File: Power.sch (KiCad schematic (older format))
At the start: 13 parts, among them P1 24 Pin Mini-Fit Jr, SW1 Power Switch

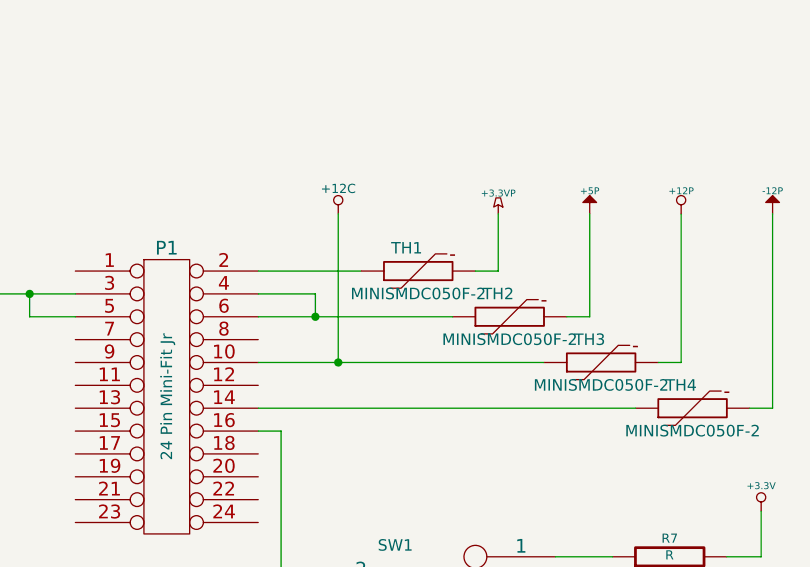
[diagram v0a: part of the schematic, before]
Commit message: Layout sessions 1-4.
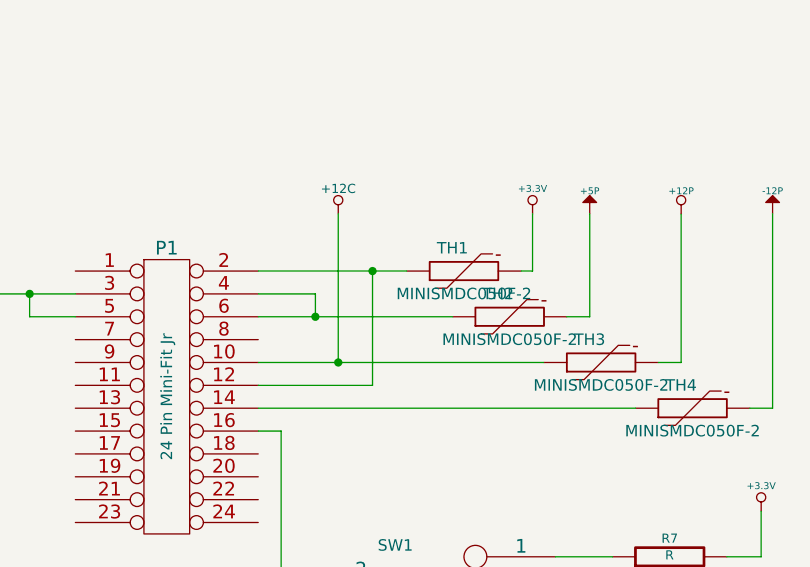
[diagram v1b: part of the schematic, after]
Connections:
- net +3.3VP is gone; now on net +3.3V: TH1.2
- net at P1.12 (P12): now also P1.2 (P2), TH1.1
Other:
- moved on the sheet: TH1
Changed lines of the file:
@@
 $EndComp
 Wire Wire Line
-	3250 2550 3700 2550
-Wire Wire Line
-	4200 2550 4300 2550
-Wire Wire Line
-	4300 2550 4300 2300
+	3250 2550 3900 2550
+Wire Wire Line
+	4400 2550 4450 2550
+Wire Wire Line
+	4450 2550 4450 2300
 Wire Wire Line
 	3250 2650 3500 2650
@@
 L THERMISTOR TH1
 U 1 1 52F96A4C
-P 3950 2550
-F 0 "TH1" V 4050 2600 50  0000 C CNN
-F 1 "MINISMDC050F-2" V 3850 2550 50  0000 C CNN
-F 2 "" H 3950 2550 60  0000 C CNN
-F 3 "" H 3950 2550 60  0000 C CNN
-F 4 "TE Connectivity" H 3950 2550 60  0001 C CNN "MFG name"
-F 5 "MINISMDC050F-2" H 3950 2550 60  0001 C CNN "MFG Part Number"
-	1    3950 2550
-	0    -1   -1   0
-$EndComp
-Wire Wire Line
-	3600 2950 3600 2300
+P 4150 2550
+F 0 "TH1" V 4250 2600 50  0000 C CNN
+F 1 "MINISMDC050F-2" V 4050 2550 50  0000 C CNN
+F 2 "" H 4150 2550 60  0000 C CNN
+F 3 "" H 4150 2550 60  0000 C CNN
+F 4 "TE Connectivity" H 4150 2550 60  0001 C CNN "MFG name"
+F 5 "MINISMDC050F-2" H 4150 2550 60  0001 C CNN "MFG Part Number"
+	1    4150 2550
+	0    -1   -1   0
+$EndComp
 Connection ~ 3600 2950
 $Comp
@@
 F 3 "" H 4700 2300 60  0000 C CNN
 	1    4700 2300
-	1    0    0    -1
-$EndComp
-$Comp
-L +3.3VP #PWR014
-U 1 1 5302613A
-P 4300 2300
-F 0 "#PWR014" H 4350 2330 20  0001 C CNN
-F 1 "+3.3VP" H 4300 2390 30  0000 C CNN
-F 2 "" H 4300 2300 60  0000 C CNN
-F 3 "" H 4300 2300 60  0000 C CNN
-	1    4300 2300
 	1    0    0    -1
 $EndComp
@@
 	0    1    1    0
 $EndComp
+$Comp
+L +3.3V #PWR014
+U 1 1 53123FE6
+P 4450 2300
+F 0 "#PWR014" H 4450 2260 30  0001 C CNN
+F 1 "+3.3V" H 4450 2410 30  0000 C CNN
+F 2 "" H 4450 2300 60  0000 C CNN
+F 3 "" H 4450 2300 60  0000 C CNN
+	1    4450 2300
+	1    0    0    -1
+$EndComp
+Wire Wire Line
+	3250 3050 3750 3050
+Wire Wire Line
+	3750 3050 3750 2550
+Connection ~ 3750 2550
+Wire Wire Line
+	3600 2300 3600 2950
 $EndSCHEMATC
